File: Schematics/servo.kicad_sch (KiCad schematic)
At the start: 1 part, among them M1 Motor_Servo

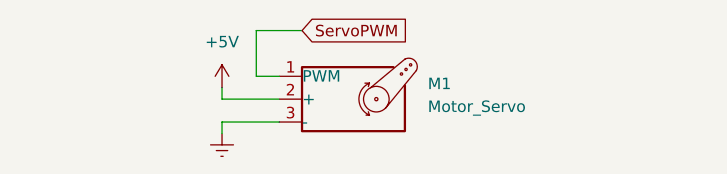
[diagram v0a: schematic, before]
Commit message: PCB
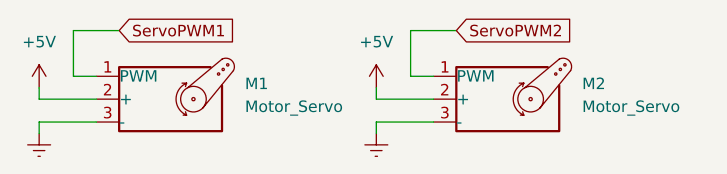
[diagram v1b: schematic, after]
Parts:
- added M2: Motor_Servo, SFRFootprints:Servo, symbol Motor:Motor_Servo
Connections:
- net +5V: now also M2.2 (+)
- net Earth: now also M2.3 (-)
- net ServoPWM renamed ServoPWM1
- new net ServoPWM2: M2.1 (PWM)
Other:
- moved on the sheet: M1
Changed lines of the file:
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@@
 (kicad_sch (version 20211123) (generator eeschema)
   (paper "A4")
-  (wire (pts (xy 137.16 102.87) (xy 137.16 101.6))
+  (wire (pts (xy 116.84 102.87) (xy 116.84 101.6))
     (stroke (width 0) (type default) (color 0 0 0 0))
   )
-  (wire (pts (xy 143.51 100.33) (xy 140.97 100.33))
+  (wire (pts (xy 160.655 100.33) (xy 158.115 100.33))
     (stroke (width 0) (type default) (color 0 0 0 0))
   )
-  (wire (pts (xy 140.97 100.33) (xy 140.97 95.25))
+  (wire (pts (xy 158.115 95.25) (xy 163.195 95.25))
     (stroke (width 0) (type default) (color 0 0 0 0))
   )
-  (wire (pts (xy 143.51 105.41) (xy 137.16 105.41))
+  (wire (pts (xy 158.115 100.33) (xy 158.115 95.25))
     (stroke (width 0) (type default) (color 0 0 0 0))
   )
-  (wire (pts (xy 143.51 102.87) (xy 137.16 102.87))
+  (wire (pts (xy 123.19 100.33) (xy 120.65 100.33))
     (stroke (width 0) (type default) (color 0 0 0 0))
   )
-  (wire (pts (xy 137.16 105.41) (xy 137.16 106.68))
+  (wire (pts (xy 154.305 105.41) (xy 154.305 106.68))
     (stroke (width 0) (type default) (color 0 0 0 0))
   )
-  (wire (pts (xy 140.97 95.25) (xy 146.05 95.25))
+  (wire (pts (xy 120.65 100.33) (xy 120.65 95.25))
     (stroke (width 0) (type default) (color 0 0 0 0))
   )
-  (global_label "ServoPWM" (shape input) (at 146.05 95.25 0) (fields_autoplaced)
+  (wire (pts (xy 123.19 105.41) (xy 116.84 105.41))
+    (stroke (width 0) (type default) (color 0 0 0 0))
+  )
+  (wire (pts (xy 154.305 102.87) (xy 154.305 101.6))
+    (stroke (width 0) (type default) (color 0 0 0 0))
+  )
+  (wire (pts (xy 160.655 105.41) (xy 154.305 105.41))
+    (stroke (width 0) (type default) (color 0 0 0 0))
+  )
+  (wire (pts (xy 160.655 102.87) (xy 154.305 102.87))
+    (stroke (width 0) (type default) (color 0 0 0 0))
+  )
+  (wire (pts (xy 123.19 102.87) (xy 116.84 102.87))
+    (stroke (width 0) (type default) (color 0 0 0 0))
+  )
+  (wire (pts (xy 116.84 105.41) (xy 116.84 106.68))
+    (stroke (width 0) (type default) (color 0 0 0 0))
+  )
+  (wire (pts (xy 120.65 95.25) (xy 125.73 95.25))
+    (stroke (width 0) (type default) (color 0 0 0 0))
+  )
+  (global_label "ServoPWM1" (shape input) (at 125.73 95.25 0) (fields_autoplaced)
     (effects (font (size 1.27 1.27)) (justify left))
-    (property "Intersheet References" "${INTERSHEET_REFS}" (id 0) (at 157.8369 95.1706 0)
+    (property "Intersheet References" "${INTERSHEET_REFS}" (id 0) (at 138.7264 95.1706 0)
       (effects (font (size 1.27 1.27)) (justify left) hide)
     )
   )
-  (symbol (lib_id "power:+5V") (at 137.16 101.6 0) (unit 1)
+  (global_label "ServoPWM2" (shape input) (at 163.195 95.25 0) (fields_autoplaced)
+    (effects (font (size 1.27 1.27)) (justify left))
+    (property "Intersheet References" "${INTERSHEET_REFS}" (id 0) (at 176.1914 95.1706 0)
+      (effects (font (size 1.27 1.27)) (justify left) hide)
+    )
+  )
+  (symbol (lib_id "power:Earth") (at 154.305 106.68 0) (unit 1)
     (in_bom yes) (on_board yes) (fields_autoplaced)
-    (property "Reference" "#PWR021" (id 0) (at 137.16 105.41 0)
+    (property "Reference" "#PWR0102" (id 0) (at 154.305 113.03 0)
       (effects (font (size 1.27 1.27)) hide)
     )
-    (property "Value" "+5V" (id 1) (at 137.16 96.52 0))
-    (property "Footprint" "" (id 2) (at 137.16 101.6 0)
+    (property "Value" "Earth" (id 1) (at 154.305 110.49 0)
       (effects (font (size 1.27 1.27)) hide)
     )
-    (property "Datasheet" "" (id 3) (at 137.16 101.6 0)
+    (property "Footprint" "" (id 2) (at 154.305 106.68 0)
+      (effects (font (size 1.27 1.27)) hide)
+    )
+    (property "Datasheet" "~" (id 3) (at 154.305 106.68 0)
       (effects (font (size 1.27 1.27)) hide)
     )
     (pin "1")
   )
-  (symbol (lib_id "power:Earth") (at 137.16 106.68 0) (unit 1)
+  (symbol (lib_id "power:+5V") (at 116.84 101.6 0) (unit 1)
     (in_bom yes) (on_board yes) (fields_autoplaced)
-    (property "Reference" "#PWR022" (id 0) (at 137.16 113.03 0)
+    (property "Reference" "#PWR021" (id 0) (at 116.84 105.41 0)
       (effects (font (size 1.27 1.27)) hide)
     )
-    (property "Value" "Earth" (id 1) (at 137.16 110.49 0)
+    (property "Value" "+5V" (id 1) (at 116.84 96.52 0))
+    (property "Footprint" "" (id 2) (at 116.84 101.6 0)
       (effects (font (size 1.27 1.27)) hide)
     )
-    (property "Footprint" "" (id 2) (at 137.16 106.68 0)
-      (effects (font (size 1.27 1.27)) hide)
-    )
-    (property "Datasheet" "~" (id 3) (at 137.16 106.68 0)
+    (property "Datasheet" "" (id 3) (at 116.84 101.6 0)
       (effects (font (size 1.27 1.27)) hide)
     )
     (pin "1")
   )
-  (symbol (lib_id "Motor:Motor_Servo") (at 151.13 102.87 0) (unit 1)
+  (symbol (lib_id "Motor:Motor_Servo") (at 168.275 102.87 0) (unit 1)
     (in_bom yes) (on_board yes) (fields_autoplaced)
-    (property "Reference" "M1" (id 0) (at 160.02 101.1665 0)
+    (property "Reference" "M2" (id 0) (at 177.165 101.1665 0)
       (effects (font (size 1.27 1.27)) (justify left))
     )
-    (property "Value" "Motor_Servo" (id 1) (at 160.02 103.7065 0)
+    (property "Value" "Motor_Servo" (id 1) (at 177.165 103.7065 0)
       (effects (font (size 1.27 1.27)) (justify left))
     )
-    (property "Footprint" "SFRFootprints:Servo" (id 2) (at 151.13 107.696 0)
+    (property "Footprint" "SFRFootprints:Servo" (id 2) (at 168.275 107.696 0)
       (effects (font (size 1.27 1.27)) hide)
     )
-    (property "Datasheet" "http://forums.parallax.com/uploads/attachments/46831/74481.png" (id 3) (at 151.13 107.696 0)
+    (property "Datasheet" "http://forums.parallax.com/uploads/attachments/46831/74481.png" (id 3) (at 168.275 107.696 0)
       (effects (font (size 1.27 1.27)) hide)
     )
+    (pin "1")
+    (pin "2")
+    (pin "3")
+  )
+  (symbol (lib_id "power:Earth") (at 116.84 106.68 0) (unit 1)
+    (in_bom yes) (on_board yes) (fields_autoplaced)
+    (property "Reference" "#PWR022" (id 0) (at 116.84 113.03 0)
+      (effects (font (size 1.27 1.27)) hide)
+    )
+    (property "Value" "Earth" (id 1) (at 116.84 110.49 0)
+      (effects (font (size 1.27 1.27)) hide)
+    )
+    (property "Footprint" "" (id 2) (at 116.84 106.68 0)
+      (effects (font (size 1.27 1.27)) hide)
+    )
+    (property "Datasheet" "~" (id 3) (at 116.84 106.68 0)
+      (effects (font (size 1.27 1.27)) hide)
+    )
+    (pin "1")
+  )
+  (symbol (lib_id "power:+5V") (at 154.305 101.6 0) (unit 1)
+    (in_bom yes) (on_board yes) (fields_autoplaced)
+    (property "Reference" "#PWR0103" (id 0) (at 154.305 105.41 0)
+      (effects (font (size 1.27 1.27)) hide)
+    )
+    (property "Value" "+5V" (id 1) (at 154.305 96.52 0))
+    (property "Footprint" "" (id 2) (at 154.305 101.6 0)
+      (effects (font (size 1.27 1.27)) hide)
+    )
+    (property "Datasheet" "" (id 3) (at 154.305 101.6 0)
+      (effects (font (size 1.27 1.27)) hide)
+    )
+    (pin "1")
+  )
+  (symbol (lib_id "Motor:Motor_Servo") (at 130.81 102.87 0) (unit 1)
+    (in_bom yes) (on_board yes) (fields_autoplaced)
+    (property "Reference" "M1" (id 0) (at 139.7 101.1665 0)
+      (effects (font (size 1.27 1.27)) (justify left))
+    )
+    (property "Value" "Motor_Servo" (id 1) (at 139.7 103.7065 0)
+      (effects (font (size 1.27 1.27)) (justify left))
+    )
+    (property "Footprint" "SFRFootprints:Servo" (id 2) (at 130.81 107.696 0)
+      (effects (font (size 1.27 1.27)) hide)
+    )
+    (property "Datasheet" "http://forums.parallax.com/uploads/attachments/46831/74481.png" (id 3) (at 130.81 107.696 0)
+      (effects (font (size 1.27 1.27)) hide)
+    )
